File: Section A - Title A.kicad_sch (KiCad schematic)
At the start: 27 parts, among them J1 10155435-00011LF, J3 691382010006, J7 691382010006, U1 ESP32-S3-WROOM-2, U6 DS3231MZ

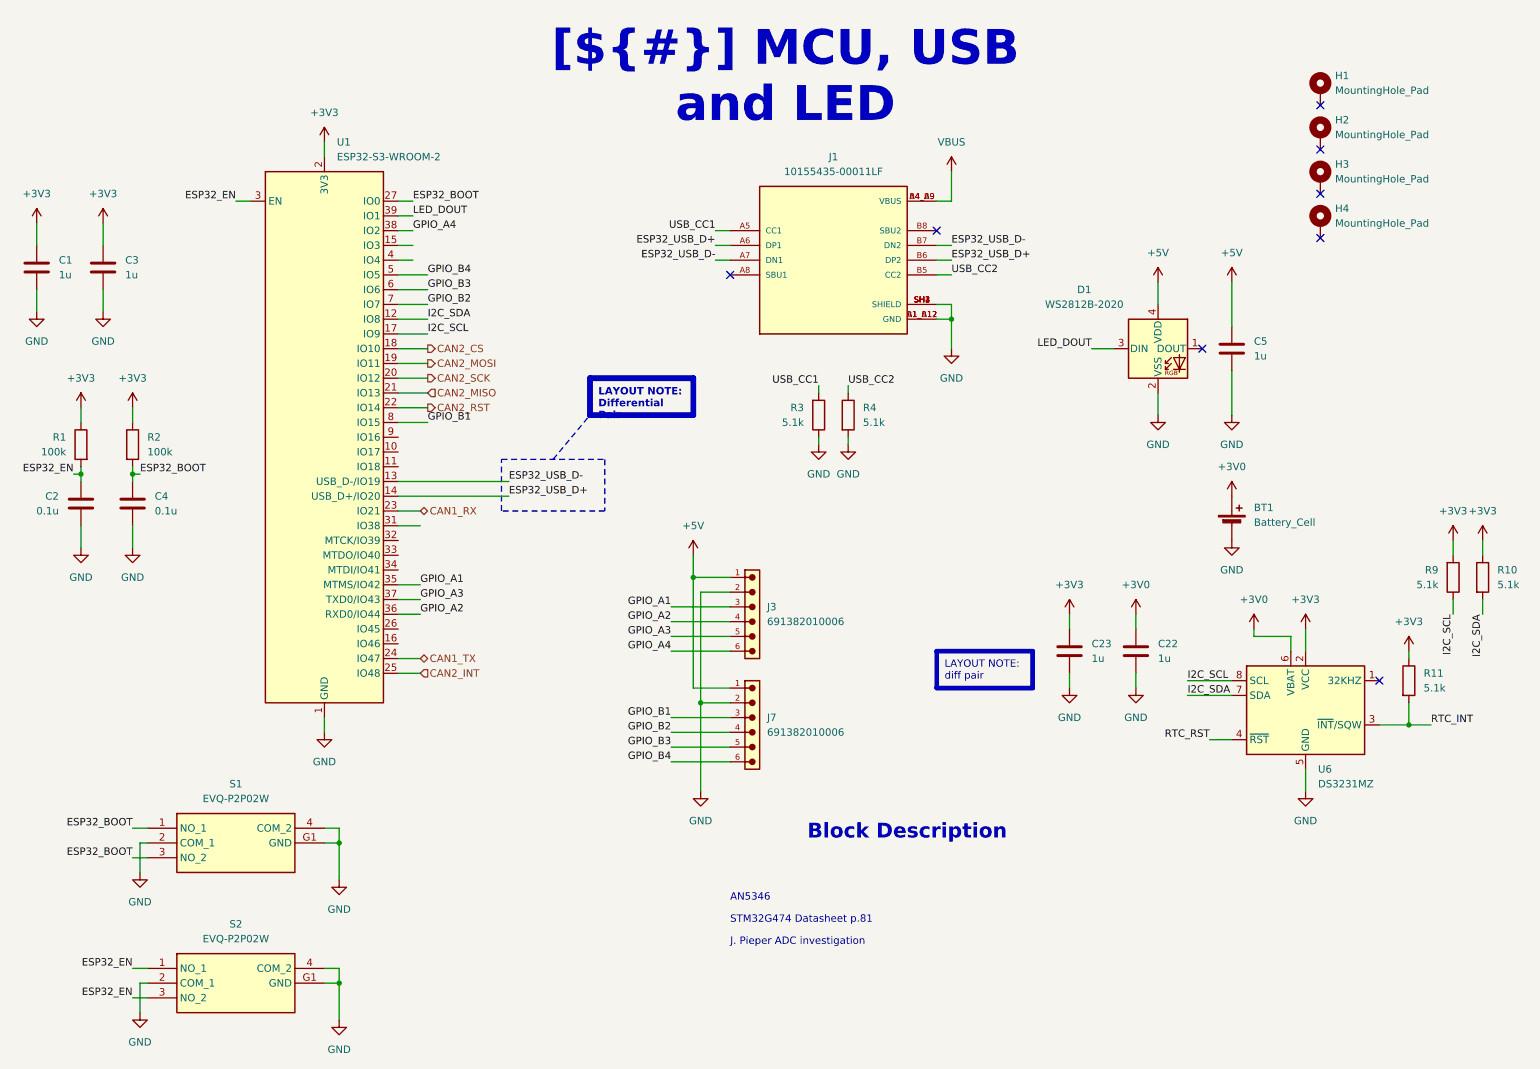
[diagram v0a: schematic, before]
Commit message: Final Changes, Updated to Checked
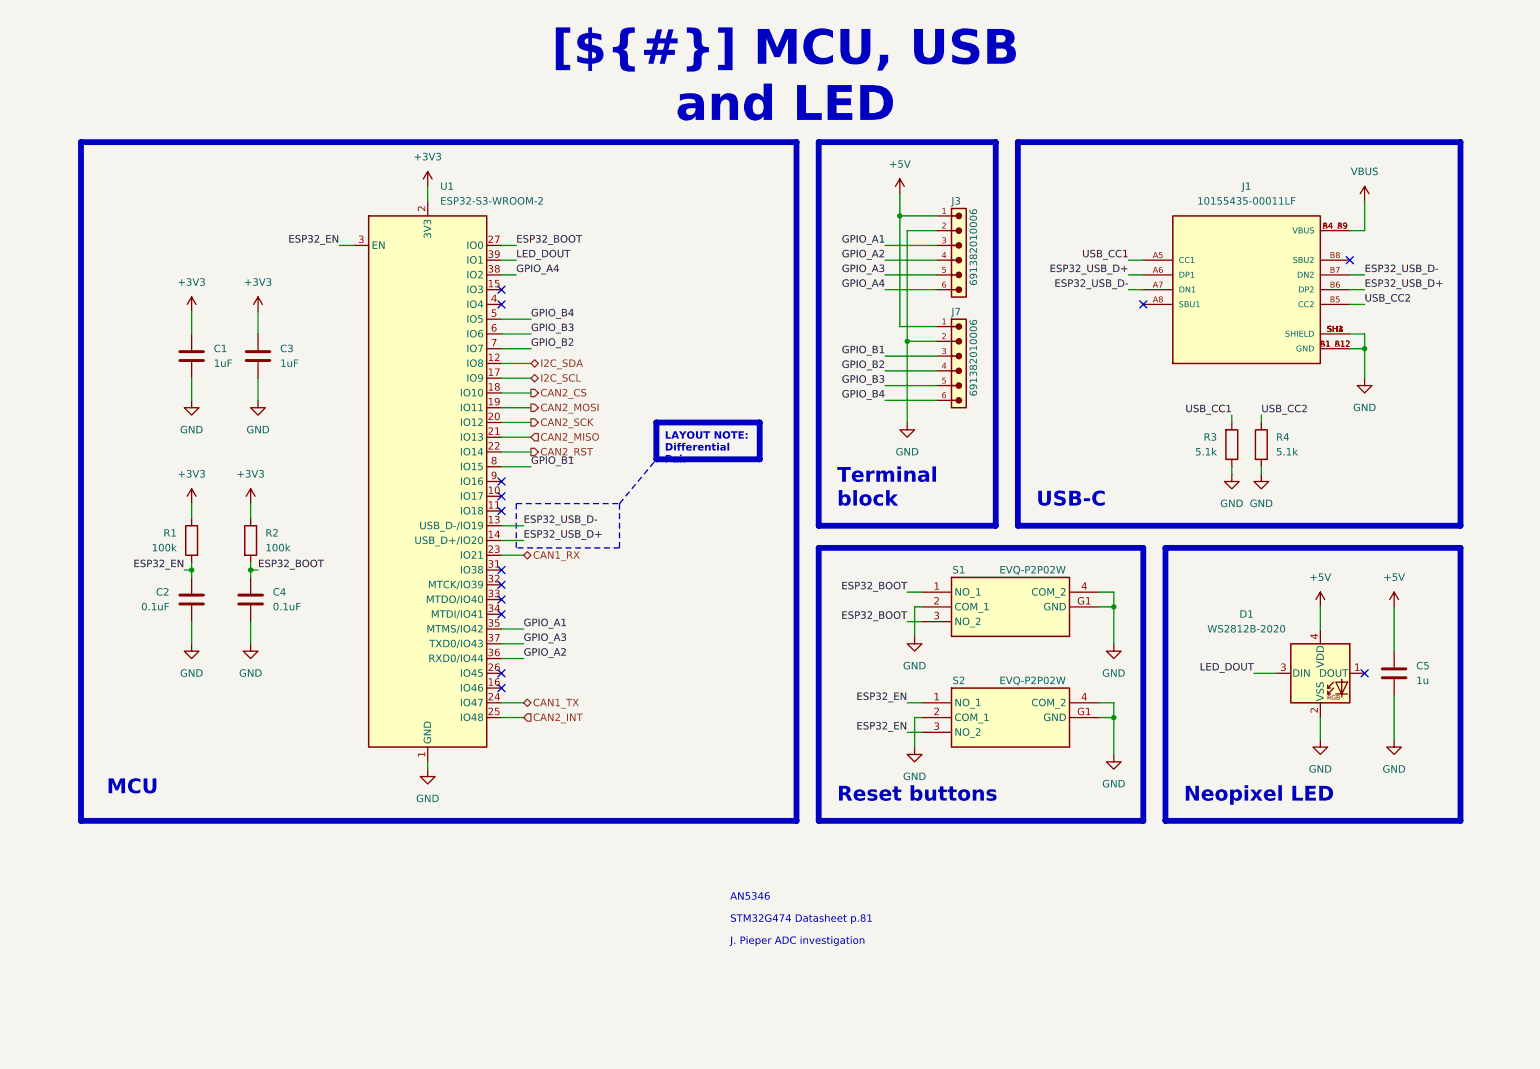
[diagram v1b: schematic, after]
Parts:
- removed BT1: Battery_Cell, Battery:BatteryHolder_MYOUNG_BS-07-A1BJ001_CR2032, symbol Device:Battery_Cell
- removed C22, C23: 1u, Capacitor_SMD:C_0603_1608Metric_Pad1.08x0.95mm_HandSolder, symbol Device:C
- removed H1, H2, H3, H4: MountingHole_Pad, MountingHole:MountingHole_3.2mm_M3_DIN965_Pad, symbol Mechanical:MountingHole_Pad
- removed R10, R11, R9: 5.1k, Resistor_SMD:R_0603_1608Metric_Pad0.98x0.95mm_HandSolder, symbol Device:R
- removed U6: DS3231MZ, Package_SO:SOIC-8_3.9x4.9mm_P1.27mm, symbol Timer_RTC:DS3231MZ
- C1, C3: value 1u -> 1uF
- C2, C4: value 0.1u -> 0.1uF
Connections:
- no-connect marks 8 -> 14
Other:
- moved on the sheet: C1, C2, C3, C4, C5, D1, J1, J3, J7, R1, R2, R3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
